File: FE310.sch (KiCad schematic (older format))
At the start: 45 parts, among them Q1 SSM3K35AMFV, Q2 SSM3K35AMFV, SW1 NP_TACTILE_SWITCH, SW2 TACTILE_SWITCH, U1 FE310-G000, U2 IS25LP128-JBLE, Y1 16MHz

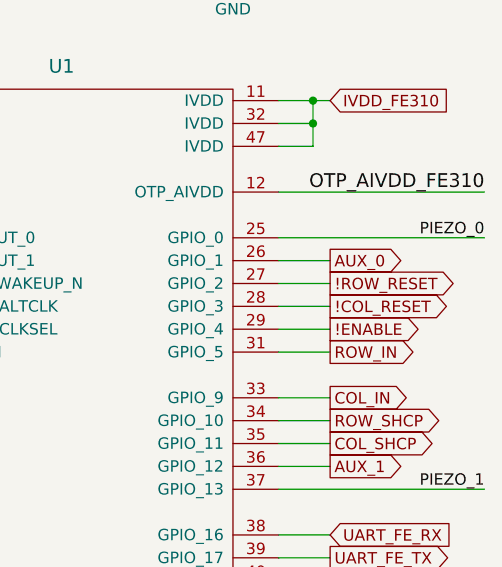
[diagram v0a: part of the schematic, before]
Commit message: automated commit
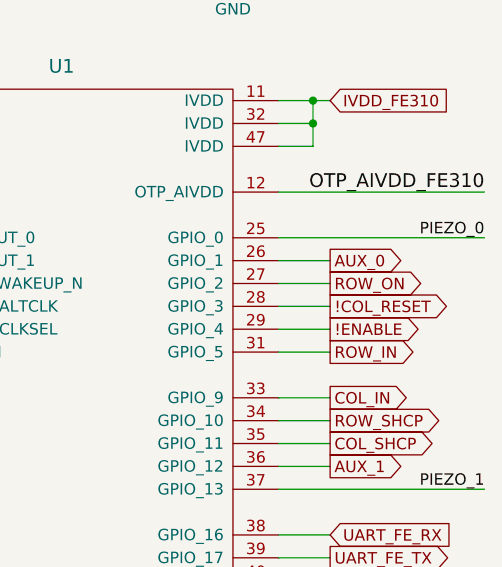
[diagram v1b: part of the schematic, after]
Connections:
- net labels added: ROW_ON
- net labels removed: !ROW_RESET
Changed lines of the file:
@@
 IVDD_FE310
 Text GLabel 9550 3625 2    50   Output ~ 0
-!ROW_RESET
+ROW_ON
 Text GLabel 9550 3725 2    50   Output ~ 0
 !COL_RESET
